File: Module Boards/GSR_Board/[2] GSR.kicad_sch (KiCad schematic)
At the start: 26 parts, among them U1 AD8236ARMZ-R7, U2 LTC2064IDD#PBF, U3 MAX5419LETA+T, U4 MAX5419LETA+T

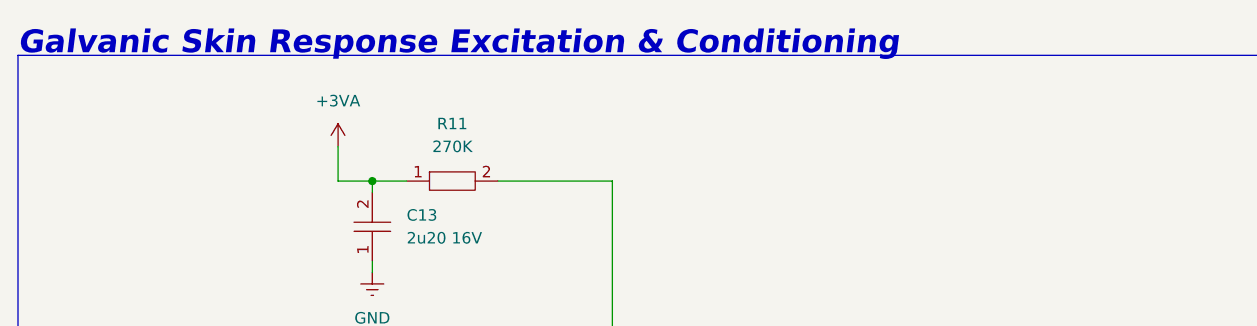
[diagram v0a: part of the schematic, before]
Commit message: Finished Routing of GSR Board
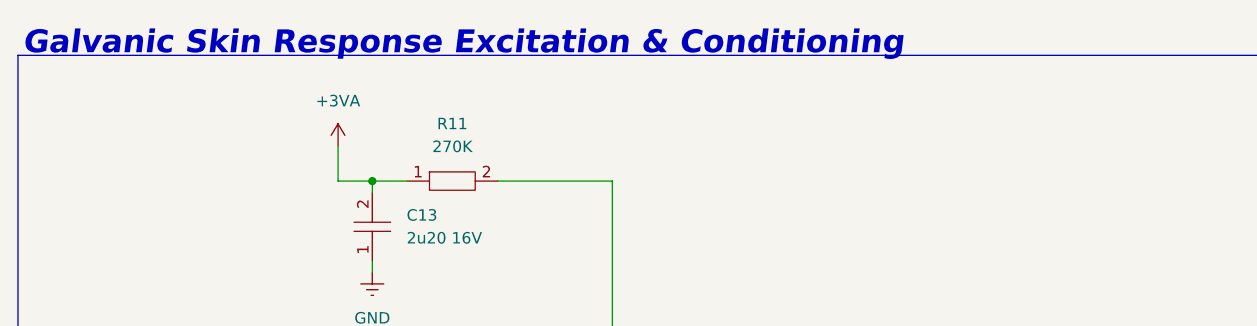
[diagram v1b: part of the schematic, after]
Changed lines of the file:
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@@
 	(text "Galvanic Skin Response Excitation & Conditioning"
 		(exclude_from_sim no)
-		(at 22.86 21.59 0)
+		(at 23.368 21.59 0)
 		(effects
 			(font
